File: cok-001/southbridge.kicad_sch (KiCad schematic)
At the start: 1 part, among them U3001 CXD29

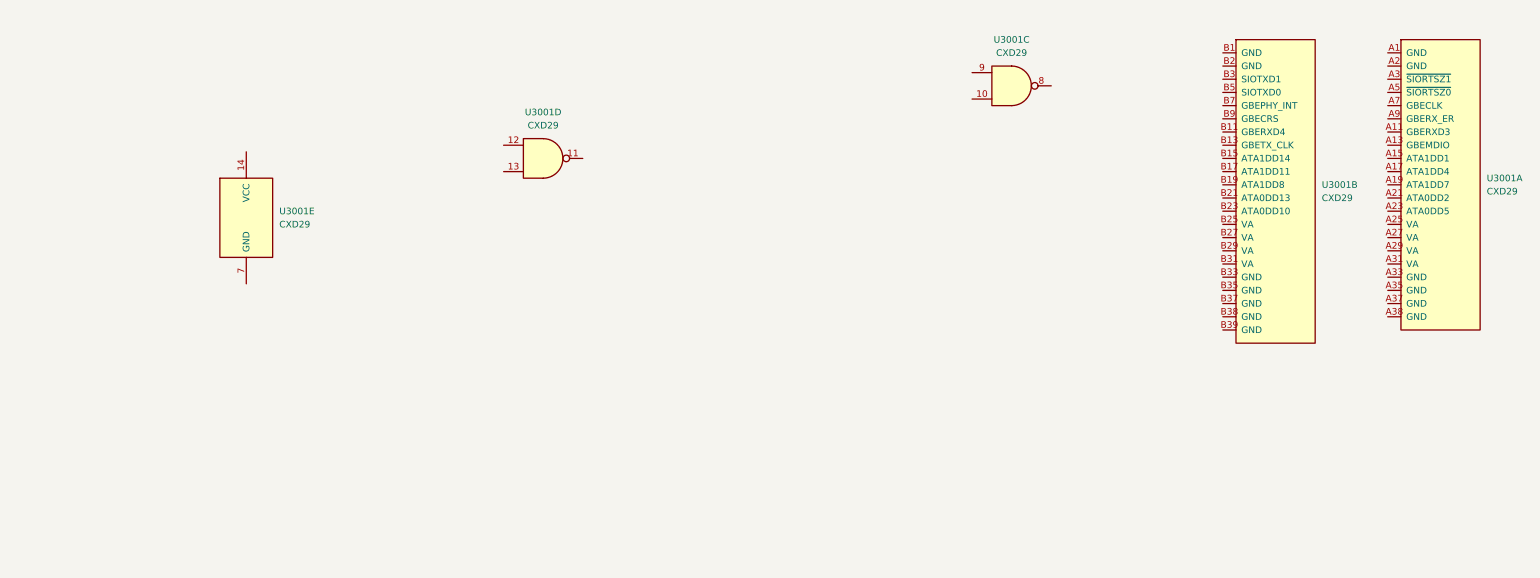
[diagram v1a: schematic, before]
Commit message: southbridge
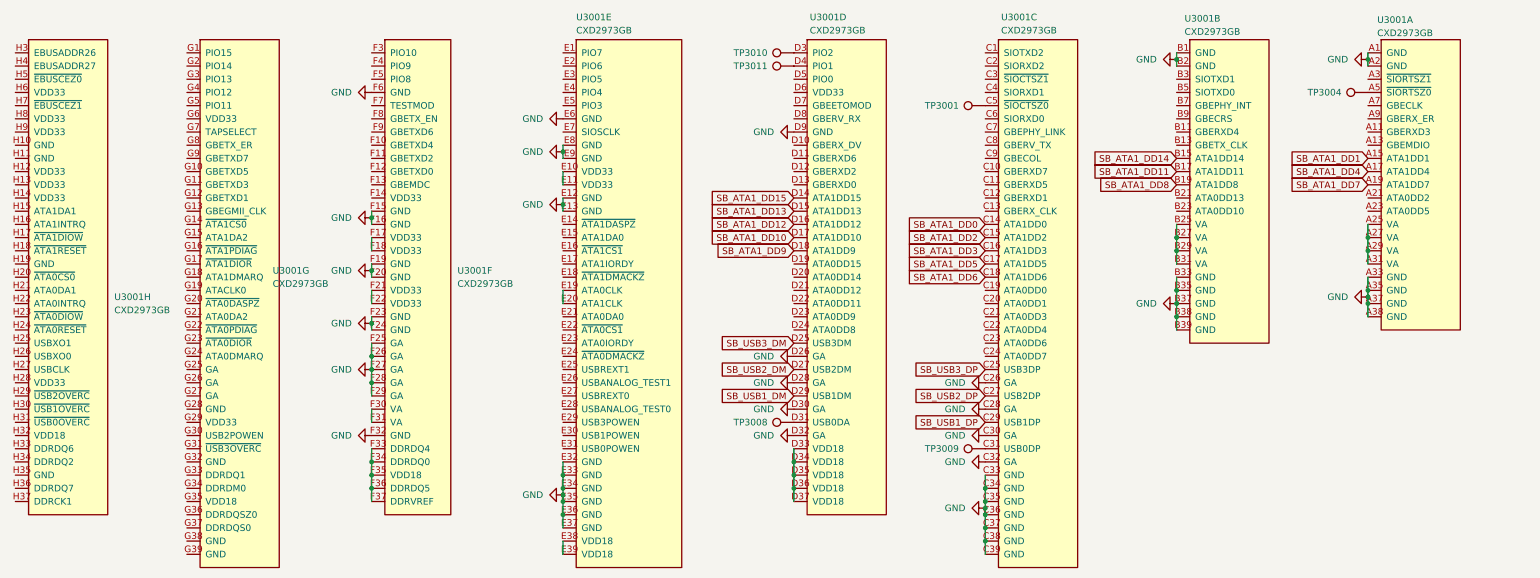
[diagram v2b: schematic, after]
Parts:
- removed U3001: CXD29, PS3:SouthBridge, symbol PS3:CXD29
- added TP3001, TP3004, TP3008, TP3009, TP3010, TP3011: TestPoint, TestPoint:TestPoint_Pad_1.0x1.0mm, symbol Connector:TestPoint
- added U3001: CXD2973GB, PS3:SouthBridge, symbol PS3:CXD2973GB
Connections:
- new net: TP3010.1, U3001.D3 (PIO2)
- new net: U3001.F17 (VDD33), U3001.F18 (VDD33)
- new net: U3001.F21 (VDD33), U3001.F22 (VDD33)
- new net: U3001.F30 (VA), U3001.F31 (VA)
- new net: U3001.F33 (DDRDQ4), U3001.F34 (DDRDQ0), U3001.F35 (VDD18), U3001.F36 (DDRDQ5), U3001.F37 (DDRVREF)
- new net: U3001.B25 (VA), U3001.B27 (VA), U3001.B29 (VA), U3001.B31 (VA)
- new net: U3001.A25 (VA), U3001.A27 (VA), U3001.A29 (VA), U3001.A31 (VA)
- new net: TP3004.1, U3001.A5 (~{SIORTSZ0})
- new net: TP3001.1, U3001.C5 (~{SIOCTSZ0})
- new net: TP3008.1, U3001.D31 (USB0DA)
- new net: TP3009.1, U3001.C31 (USB0DP)
- new net: U3001.D33 (VDD18), U3001.D34 (VDD18), U3001.D35 (VDD18), U3001.D36 (VDD18), U3001.D37 (VDD18)
- new net: TP3011.1, U3001.D4 (PIO1)
- new net: U3001.E10 (VDD33), U3001.E11 (VDD33)
- new net: U3001.E19 (ATA0CLK), U3001.E20 (ATA1CLK)
- new net: U3001.E38 (VDD18), U3001.E39 (VDD18)
- new net GND: U3001.A1 (GND), U3001.A2 (GND), U3001.A33 (GND), U3001.A35 (GND), U3001.A37 (GND), U3001.A38 (GND), U3001.B1 (GND), U3001.B2 (GND), U3001.B33 (GND), U3001.B35 (GND), U3001.B37 (GND), U3001.B38 (GND), U3001.B39 (GND), U3001.C26 (GA), U3001.C28 (GA), U3001.C30 (GA), U3001.C32 (GA), U3001.C33 (GND), U3001.C34 (GND), U3001.C35 (GND), U3001.C36 (GND), U3001.C37 (GND), U3001.C38 (GND), U3001.C39 (GND), U3001.D26 (GA), U3001.D28 (GA), U3001.D30 (GA), U3001.D32 (GA), U3001.D9 (GND), U3001.E12 (GND), U3001.E13 (GND), U3001.E32 (GND), U3001.E33 (GND), U3001.E34 (GND), U3001.E35 (GND), U3001.E36 (GND), U3001.E37 (GND), U3001.E6 (GND), U3001.E8 (GND), U3001.E9 (GND), U3001.F15 (GND), U3001.F16 (GND), U3001.F19 (GND), U3001.F20 (GND), U3001.F23 (GND), U3001.F24 (GND), U3001.F25 (GA), U3001.F26 (GA), U3001.F27 (GA), U3001.F28 (GA), U3001.F29 (GA), U3001.F32 (GND), U3001.F6 (GND)
- new net SB_ATA1_DD0: U3001.C14 (ATA1DD0)
- new net SB_ATA1_DD1: U3001.A15 (ATA1DD1)
- new net SB_ATA1_DD10: U3001.D17 (ATA1DD10)
- new net SB_ATA1_DD11: U3001.B17 (ATA1DD11)
- new net SB_ATA1_DD12: U3001.D16 (ATA1DD12)
- new net SB_ATA1_DD13: U3001.D15 (ATA1DD13)
- new net SB_ATA1_DD14: U3001.B15 (ATA1DD14)
- new net SB_ATA1_DD15: U3001.D14 (ATA1DD15)
- new net SB_ATA1_DD2: U3001.C15 (ATA1DD2)
- new net SB_ATA1_DD3: U3001.C16 (ATA1DD3)
- new net SB_ATA1_DD4: U3001.A17 (ATA1DD4)
- new net SB_ATA1_DD5: U3001.C17 (ATA1DD5)
- new net SB_ATA1_DD6: U3001.C18 (ATA1DD6)
- new net SB_ATA1_DD7: U3001.A19 (ATA1DD7)
- new net SB_ATA1_DD8: U3001.B19 (ATA1DD8)
- new net SB_ATA1_DD9: U3001.D18 (ATA1DD9)
- new net SB_USB1_DM: U3001.D29 (USB1DM)
- new net SB_USB1_DP: U3001.C29 (USB1DP)
- new net SB_USB2_DM: U3001.D27 (USB2DM)
- new net SB_USB2_DP: U3001.C27 (USB2DP)
- new net SB_USB3_DM: U3001.D25 (USB3DM)
- new net SB_USB3_DP: U3001.C25 (USB3DP)

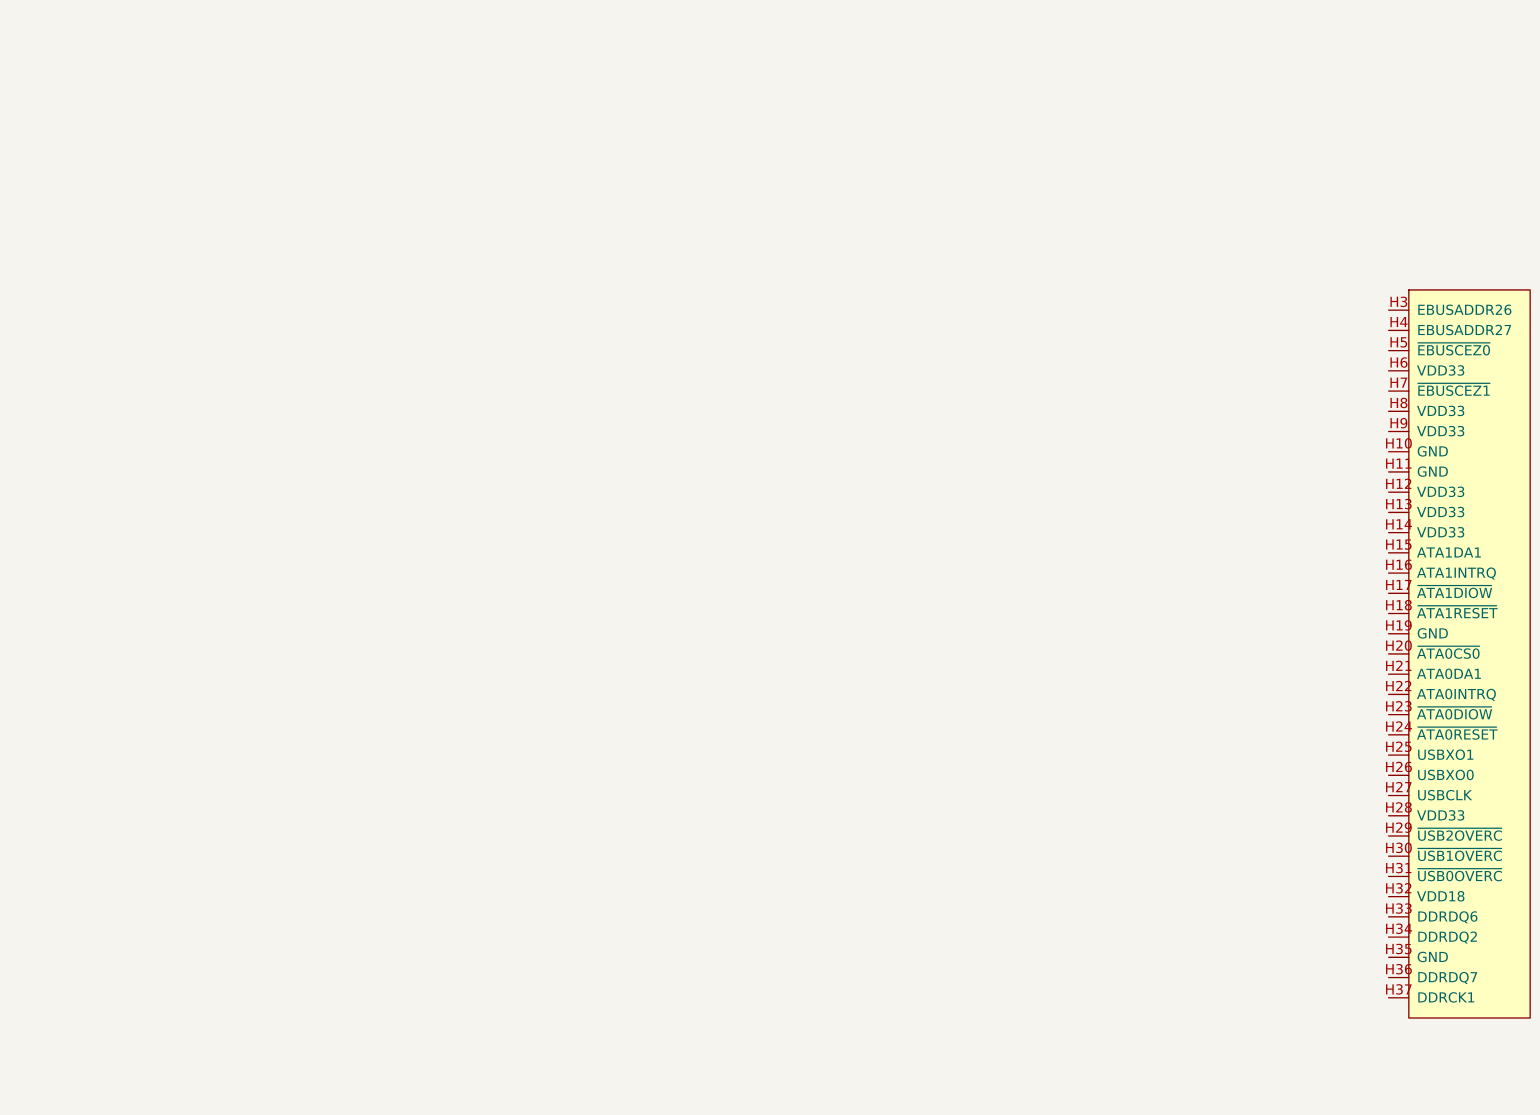
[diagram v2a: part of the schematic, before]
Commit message: L
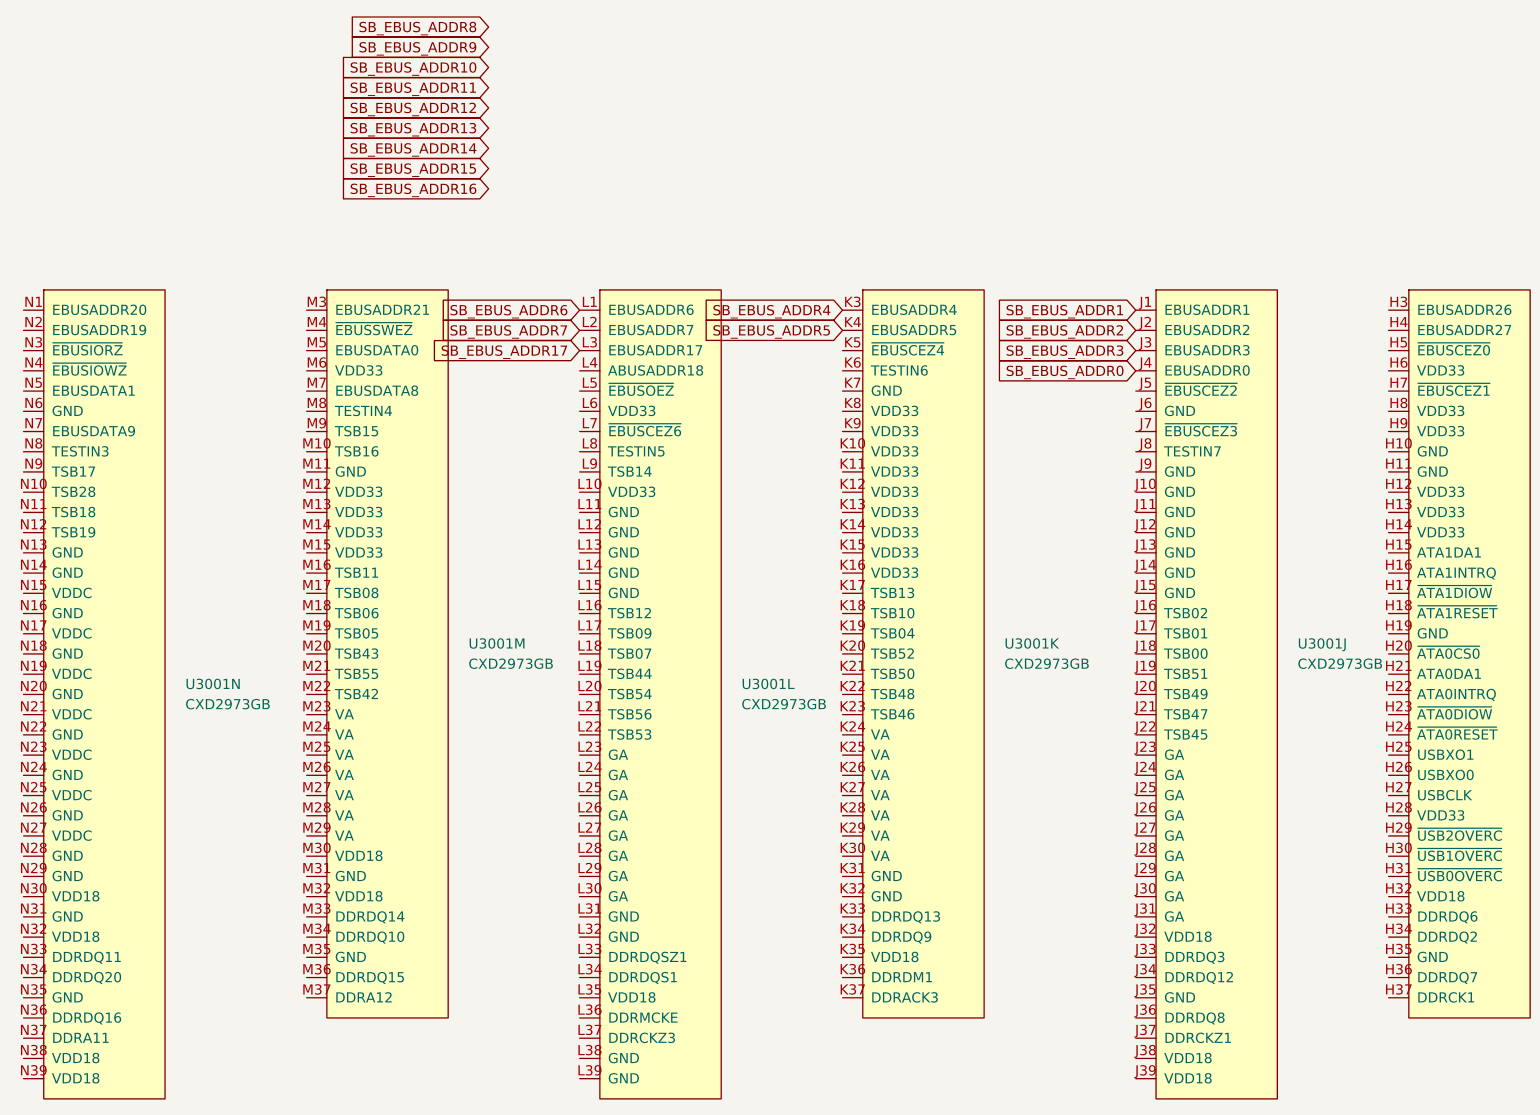
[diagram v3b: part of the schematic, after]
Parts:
- added unit 11 of U3001
- added unit 13 of U3001
- added unit 10 of U3001
- added unit 14 of U3001
- added unit 12 of U3001
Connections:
- new net SB_EBUS_ADDR0: U3001.J4 (EBUSADDR0)
- new net SB_EBUS_ADDR1: U3001.J1 (EBUSADDR1)
- new net SB_EBUS_ADDR17: U3001.L3 (EBUSADDR17)
- new net SB_EBUS_ADDR2: U3001.J2 (EBUSADDR2)
- new net SB_EBUS_ADDR3: U3001.J3 (EBUSADDR3)
- new net SB_EBUS_ADDR4: U3001.K3 (EBUSADDR4)
- new net SB_EBUS_ADDR5: U3001.K4 (EBUSADDR5)
- new net SB_EBUS_ADDR6: U3001.L1 (EBUSADDR6)
- new net SB_EBUS_ADDR7: U3001.L2 (EBUSADDR7)
